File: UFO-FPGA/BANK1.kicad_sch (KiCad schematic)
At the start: 7 parts, among them U1 ICE40HX8K-BG121

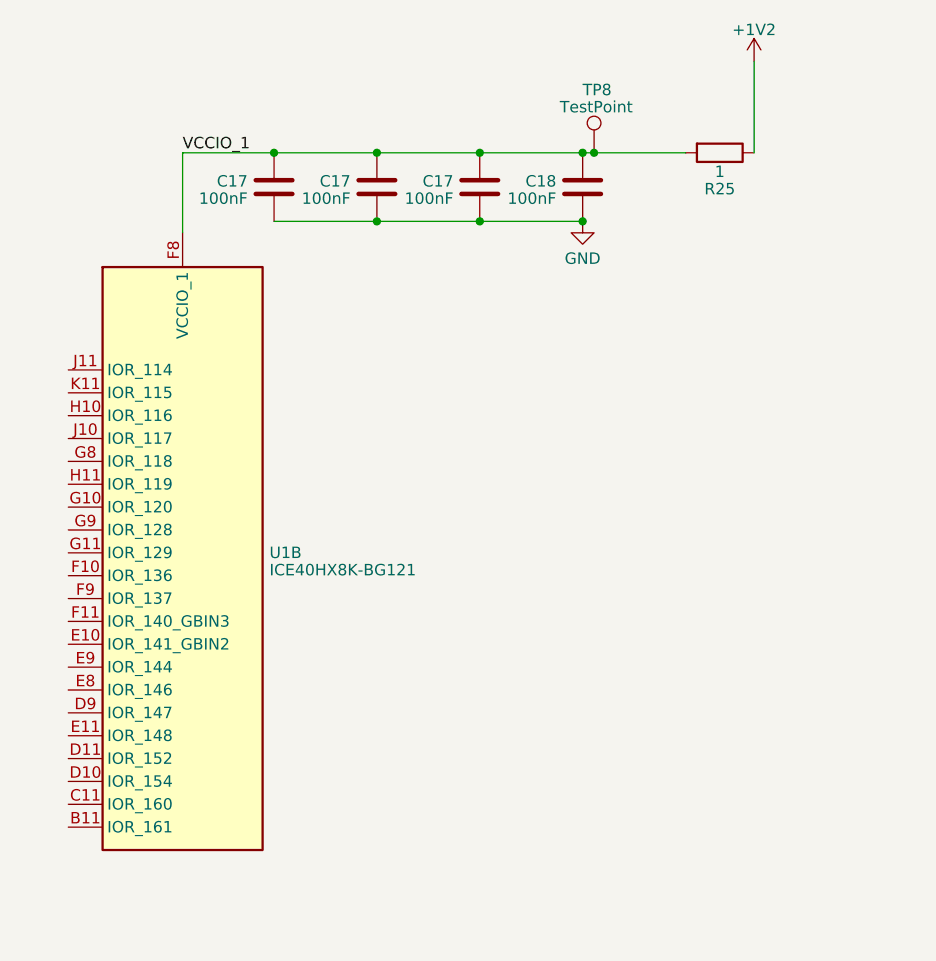
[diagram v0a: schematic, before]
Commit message: IO and power
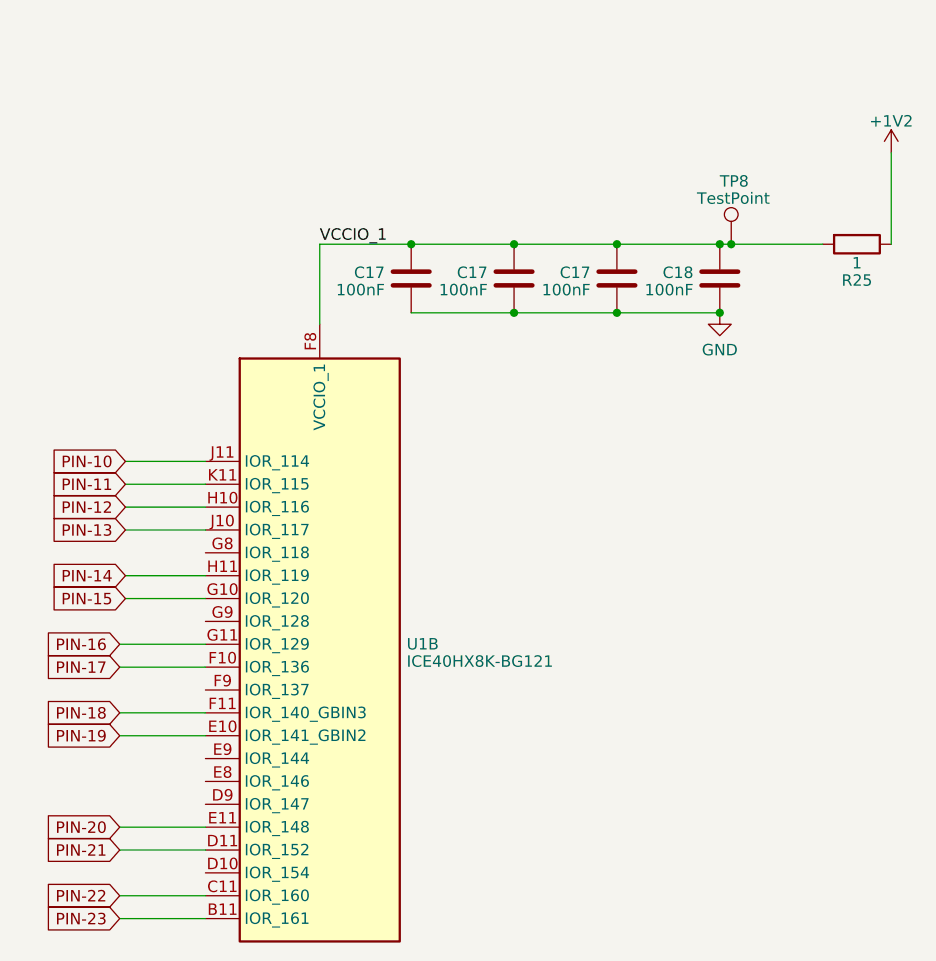
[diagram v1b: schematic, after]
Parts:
- removed C17 (x3): 100nF, symbol Device:C
- added C17 (x3): 100nF, symbol Device:C
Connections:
- net GND: now also C17.2, C17.2, C17.2
- net VCCIO_1: now also C17.1, C17.1, C17.1
- net PIN-23: now reaches U1.B11 (IOR_161)
- net PIN-22: now reaches U1.C11 (IOR_160)
- net PIN-21: now reaches U1.D11 (IOR_152)
- net PIN-19: now reaches U1.E10 (IOR_141_GBIN2)
- net PIN-20: now reaches U1.E11 (IOR_148)
- net PIN-17: now reaches U1.F10 (IOR_136)
- net PIN-18: now reaches U1.F11 (IOR_140_GBIN3)
- net PIN-15: now reaches U1.G10 (IOR_120)
- net PIN-16: now reaches U1.G11 (IOR_129)
- net PIN-12: now reaches U1.H10 (IOR_116)
- net PIN-14: now reaches U1.H11 (IOR_119)
- net PIN-13: now reaches U1.J10 (IOR_117)
- net PIN-10: now reaches U1.J11 (IOR_114)
- net PIN-11: now reaches U1.K11 (IOR_115)
